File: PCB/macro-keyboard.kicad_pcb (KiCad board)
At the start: 2 copper layers, 77.6 x 43 mm, 38 parts, among them SW1 SW_Push, SW2 SW_Push, SW3 SW_Push, SW4 SW_Push, SW5 SW_Push, SW6 SW_Push, SW7 SW_Push, SW8 SW_Push, U1 PRTR5V0U2X, U2 ATmega32U4-A, Y1 Crystal_GND24_Small

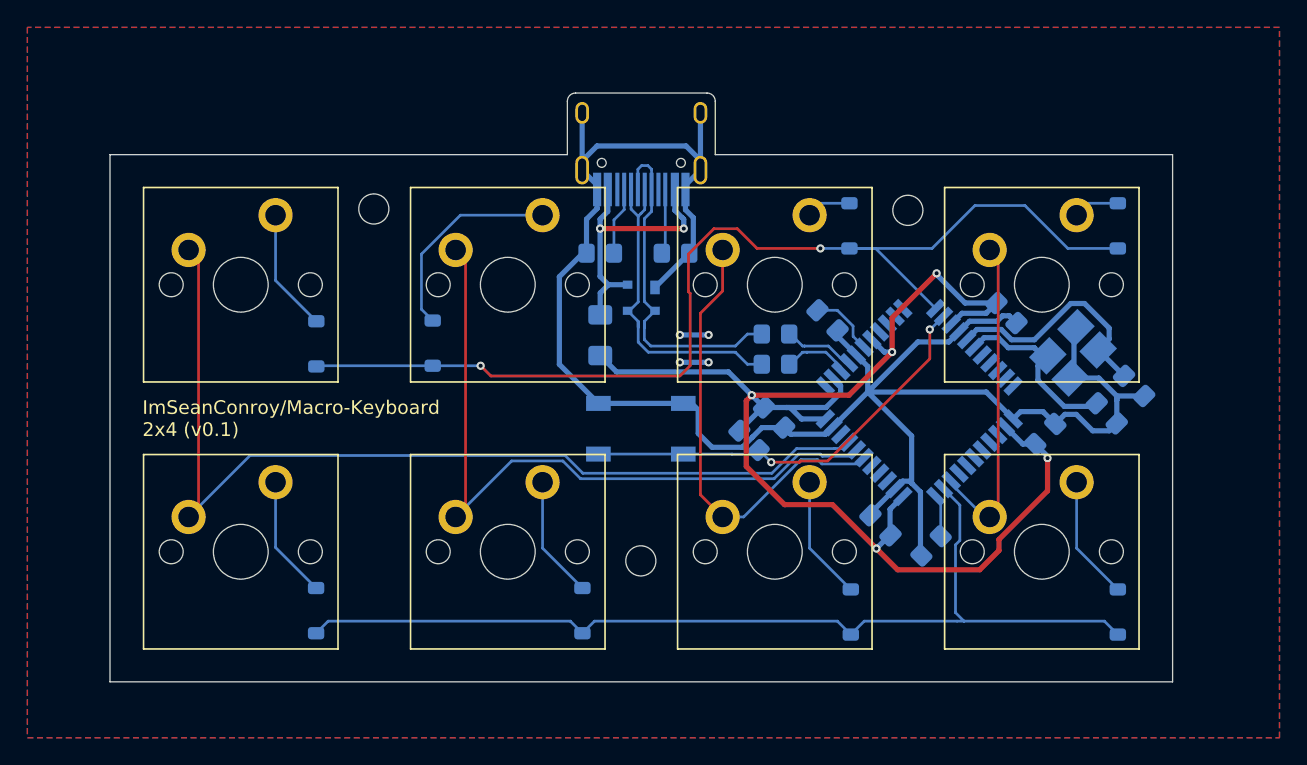
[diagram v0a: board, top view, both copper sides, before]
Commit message: Add gerber files
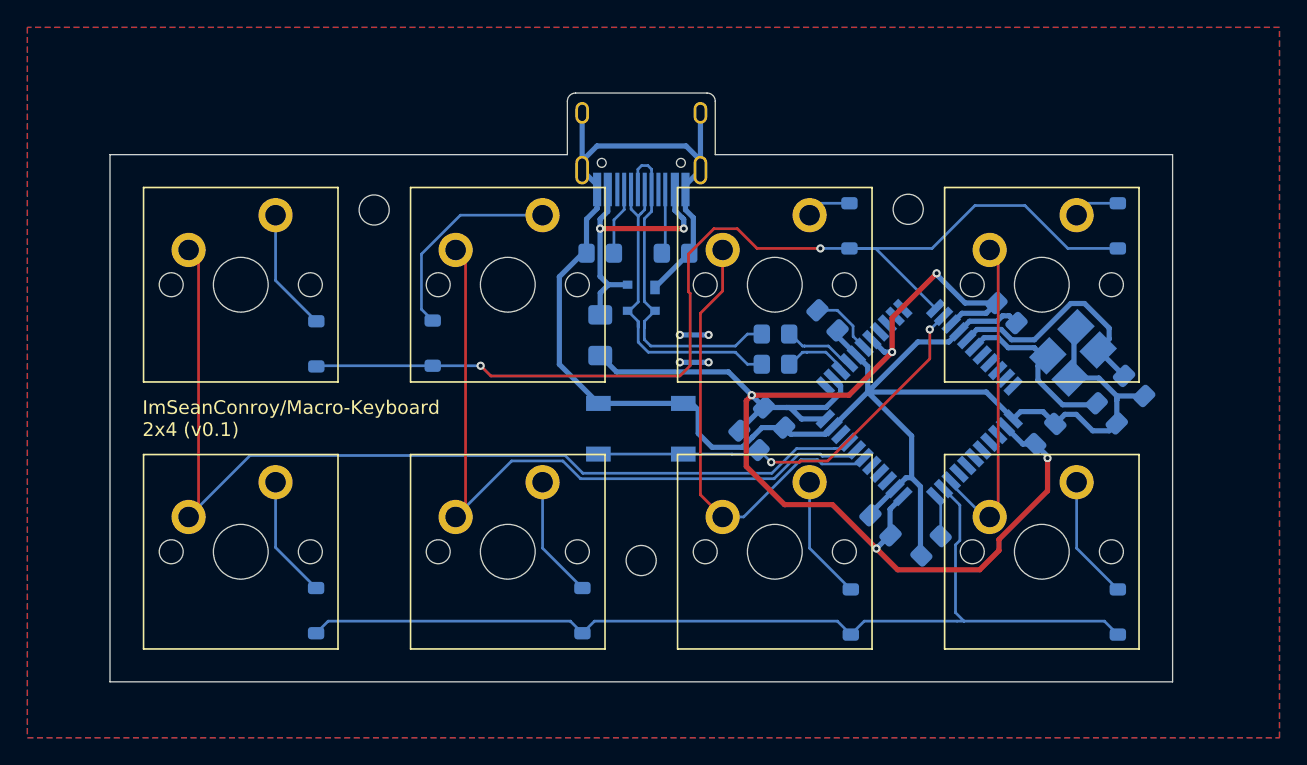
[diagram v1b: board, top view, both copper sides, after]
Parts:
- moved REF** 0.08 mm to (165.9, 83.3)
- moved REF** 0.08 mm to (126.9, 83.4)
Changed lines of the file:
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@@
 			(disableapertmacros no)
 			(usegerberextensions no)
-			(usegerberattributes yes)
-			(usegerberadvancedattributes yes)
-			(creategerberjobfile yes)
+			(usegerberattributes no)
+			(usegerberadvancedattributes no)
+			(creategerberjobfile no)
 			(dashed_line_dash_ratio 12.000000)
 			(dashed_line_gap_ratio 3.000000)
 			(svgprecision 4)
 			(plotframeref no)
-			(viasonmask no)
+			(viasonmask yes)
 			(mode 1)
 			(useauxorigin no)
@@
 			(outputformat 1)
 			(mirror no)
-			(drillshape 1)
+			(drillshape 0)
 			(scaleselection 1)
-			(outputdirectory "")
+			(outputdirectory "Fabrication/")
 		)
 	)
@@
 	(footprint "MountingHole:MountingHole_2.2mm_M2_DIN965"
 		(layer "F.Cu")
-		(at 146.4 109)
+		(at 146.425 108.975)
 		(descr "Mounting Hole 2.2mm, no annular, M2, DIN965")
 		(tags "mounting hole 2.2mm no annular m2 din965")
@@
 	(footprint "MountingHole:MountingHole_2.2mm_M2_DIN965"
 		(layer "F.Cu")
-		(at 165.9 83.4)
+		(at 165.925 83.325)
 		(descr "Mounting Hole 2.2mm, no annular, M2, DIN965")
 		(tags "mounting hole 2.2mm no annular m2 din965")
@@
 	(footprint "MountingHole:MountingHole_2.2mm_M2_DIN965"
 		(layer "F.Cu")
-		(at 126.9 83.3)
+		(at 126.925 83.375)
 		(descr "Mounting Hole 2.2mm, no annular, M2, DIN965")
 		(tags "mounting hole 2.2mm no annular m2 din965")
@@
 	)
 	(segment
+		(start 175.4 95.8)
+		(end 177.2 97.6)
+		(width 0.381)
+		(layer "B.Cu")
+		(net 2)
+	)
+	(segment
 		(start 175.724264 94.024264)
 		(end 176.123044 94.024264)
@@
 	)
 	(segment
-		(start 175.4 95.8)
-		(end 177.319 97.719)
+		(start 179.580062 97.6)
+		(end 179.689421 97.490641)
 		(width 0.381)
 		(layer "B.Cu")
@@
 	)
 	(segment
-		(start 179.461062 97.719)
-		(end 179.689421 97.490641)
+		(start 177.2 97.6)
+		(end 179.580062 97.6)
 		(width 0.381)
 		(layer "B.Cu")
@@
 	)
 	(segment
-		(start 177.319 97.719)
-		(end 179.461062 97.719)
-		(width 0.381)
-		(layer "B.Cu")
-		(net 2)
-	)
-	(segment
 		(start 175.4 94.747308)
 		(end 175.4 95.8)
@@
 	)
 	(segment
-		(start 166.029169 103.177275)
-		(end 165.515454 103.177275)
-		(width 0.381)
-		(layer "B.Cu")
-		(net 4)
-	)
-	(segment
 		(start 142.166377 86.533623)
 		(end 142.433623 86.533623)
@@
 	)
 	(segment
-		(start 166.885786 108.614214)
-		(end 166.820421 108.548849)
-		(width 0.381)
-		(layer "B.Cu")
-		(net 4)
-	)
-	(segment
 		(start 142.113623 79.786377)
 		(end 142.113623 80.463623)
@@
 	)
 	(segment
+		(start 166.820421 103.569474)
+		(end 166.175947 102.925)
+		(width 0.381)
+		(layer "B.Cu")
+		(net 4)
+	)
+	(segment
 		(start 181.156667 97.259107)
 		(end 181.156667 98.957887)
@@
 	)
 	(segment
+		(start 166.175947 99.875947)
+		(end 166.175947 102.925)
+		(width 0.381)
+		(layer "B.Cu")
+		(net 4)
+	)
+	(segment
 		(start 178.030642 92.116666)
 		(end 178.030642 95.369358)
@@
 	)
 	(segment
+		(start 166.820421 108.548849)
+		(end 166.820421 103.569474)
+		(width 0.381)
+		(layer "B.Cu")
+		(net 4)
+	)
+	(segment
 		(start 162.137429 93.9688)
 		(end 160.767246 92.598617)
@@
 	)
 	(segment
-		(start 165.515454 103.177275)
-		(end 164.965856 103.726873)
+		(start 183.156667 96.957887)
+		(end 181.157887 96.957887)
 		(width 0.381)
 		(layer "B.Cu")
@@
 	)
 	(segment
-		(start 166.820421 103.968527)
-		(end 166.175947 103.324053)
+		(start 150.753623 79.753623)
+		(end 149.7 78.7)
 		(width 0.381)
 		(layer "B.Cu")
@@
 	)
 	(segment
-		(start 183.156667 96.957887)
-		(end 181.157887 96.957887)
+		(start 163.166377 105.533623)
+		(end 163.166377 105.666377)
 		(width 0.381)
 		(layer "B.Cu")
@@
 	)
 	(segment
-		(start 150.753623 79.753623)
-		(end 149.7 78.7)
+		(start 171.627736 96.670882)
+		(end 173.592559 98.635705)
 		(width 0.381)
 		(layer "B.Cu")
@@
 	)
 	(segment
-		(start 163.166377 105.533623)
-		(end 163.166377 105.666377)
+		(start 166.175947 102.925)
+		(end 165.767729 102.925)
 		(width 0.381)
 		(layer "B.Cu")
@@
 	)
 	(segment
-		(start 171.627736 96.670882)
-		(end 173.592559 98.635705)
+		(start 162.970882 96.670882)
+		(end 166.175947 99.875947)
 		(width 0.381)
 		(layer "B.Cu")
@@
 	)
 	(segment
+		(start 166.885786 108.614214)
+		(end 166.820421 108.548849)
+		(width 0.381)
+		(layer "B.Cu")
+		(net 4)
+	)
+	(segment
 		(start 140.448123 88.251877)
 		(end 142.166377 86.533623)
@@
 	)
 	(segment
-		(start 166.175947 103.324053)
-		(end 166.175947 99.875947)
+		(start 157.350989 99.750989)
+		(end 156.867246 99.267246)
 		(width 0.381)
 		(layer "B.Cu")
@@
 	)
 	(segment
-		(start 157.350989 99.750989)
-		(end 156.867246 99.267246)
+		(start 165.767729 102.925)
+		(end 164.965856 103.726873)
 		(width 0.381)
 		(layer "B.Cu")
@@
 	)
 	(segment
-		(start 166.820421 108.548849)
-		(end 166.820421 103.968527)
-		(width 0.381)
-		(layer "B.Cu")
-		(net 4)
-	)
-	(segment
 		(start 179.4 99.5)
 		(end 180.614554 99.5)
@@
 	)
 	(segment
-		(start 166.175947 103.324053)
-		(end 166.029169 103.177275)
-		(width 0.381)
-		(layer "B.Cu")
-		(net 4)
-	)
-	(segment
 		(start 150.753623 80.463623)
 		(end 150.753623 76.283623)
@@
 		(width 0.381)
 		(layer "B.Cu")
-		(net 4)
-	)
-	(segment
-		(start 166.175947 99.875947)
-		(end 162.970882 96.670882)
-		(width 0.381)
-		(layer "B.Cu")
